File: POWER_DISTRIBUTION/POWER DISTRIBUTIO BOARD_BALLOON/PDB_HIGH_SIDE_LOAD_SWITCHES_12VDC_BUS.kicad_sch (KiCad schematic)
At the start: 20 parts, among them IC3 TPS1HB08BQPWPRQ1, IC4 TPS1HB08BQPWPRQ1

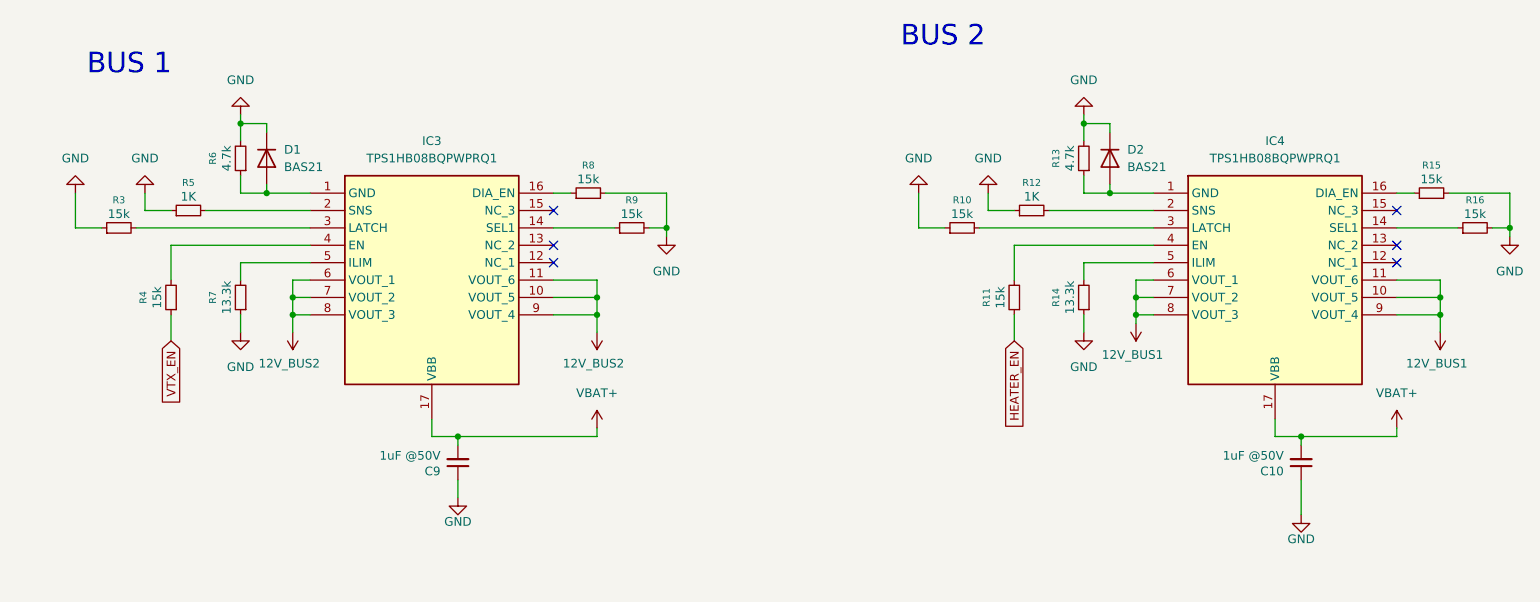
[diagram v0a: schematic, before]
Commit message: revert commit
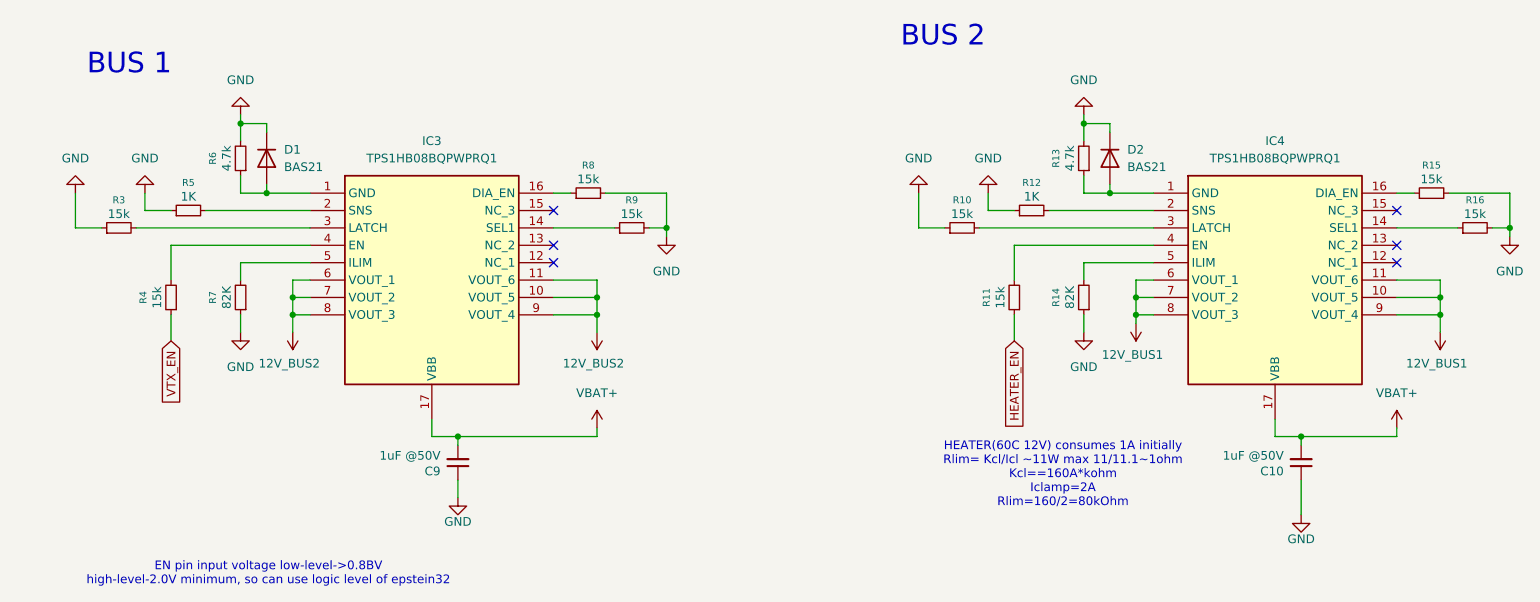
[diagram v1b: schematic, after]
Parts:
- R14, R7: value 13.3k -> 82K
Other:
- note added: "EN pin input voltage low-level->0.8BV high-level-2.0V minimum, so can use logic level of epstein32"
- note added: "HEATER(60C 12V) consumes 1A initially Rlim= Kcl/Icl ~11W max 11/11.1~1ohm Kcl==160A*kohm Iclamp=2A Rlim=160/2=80kOhm"

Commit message: test
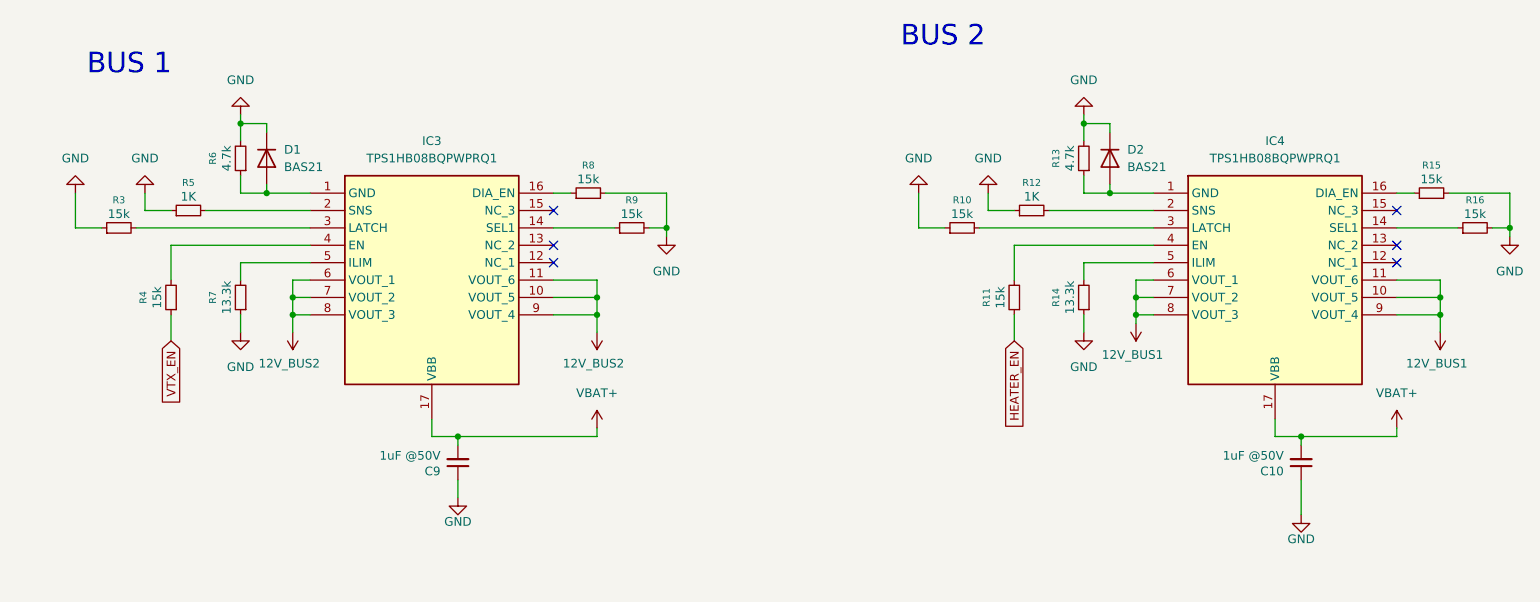
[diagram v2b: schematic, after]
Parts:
- R14, R7: value 82K -> 13.3k
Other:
- note removed: "EN pin input voltage low-level->0.8BV high-level-2.0V minimum, so can use logic level of epstein32"
- note removed: "HEATER(60C 12V) consumes 1A initially Rlim= Kcl/Icl ~11W max 11/11.1~1ohm Kcl==160A*kohm Iclamp=2A Rlim=160/2=80kOhm"
